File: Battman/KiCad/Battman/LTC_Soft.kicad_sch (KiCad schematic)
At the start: 14 parts, among them IC600 LTC6811IG-2#PBF, Q600 BCP56-16TF

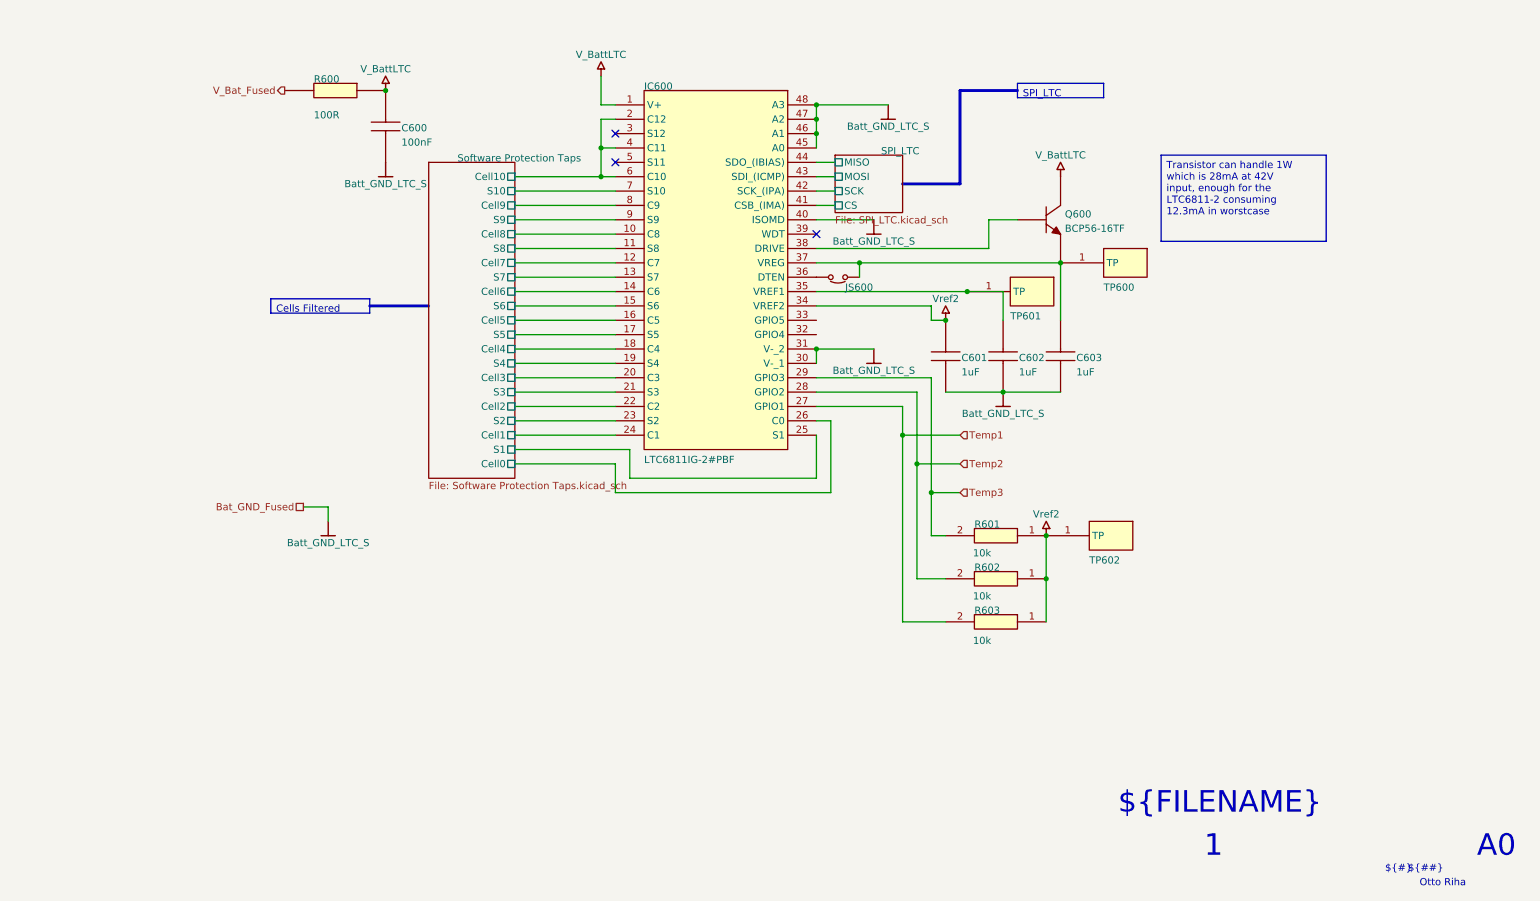
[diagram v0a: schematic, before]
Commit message: Uopdated Schematics fixed
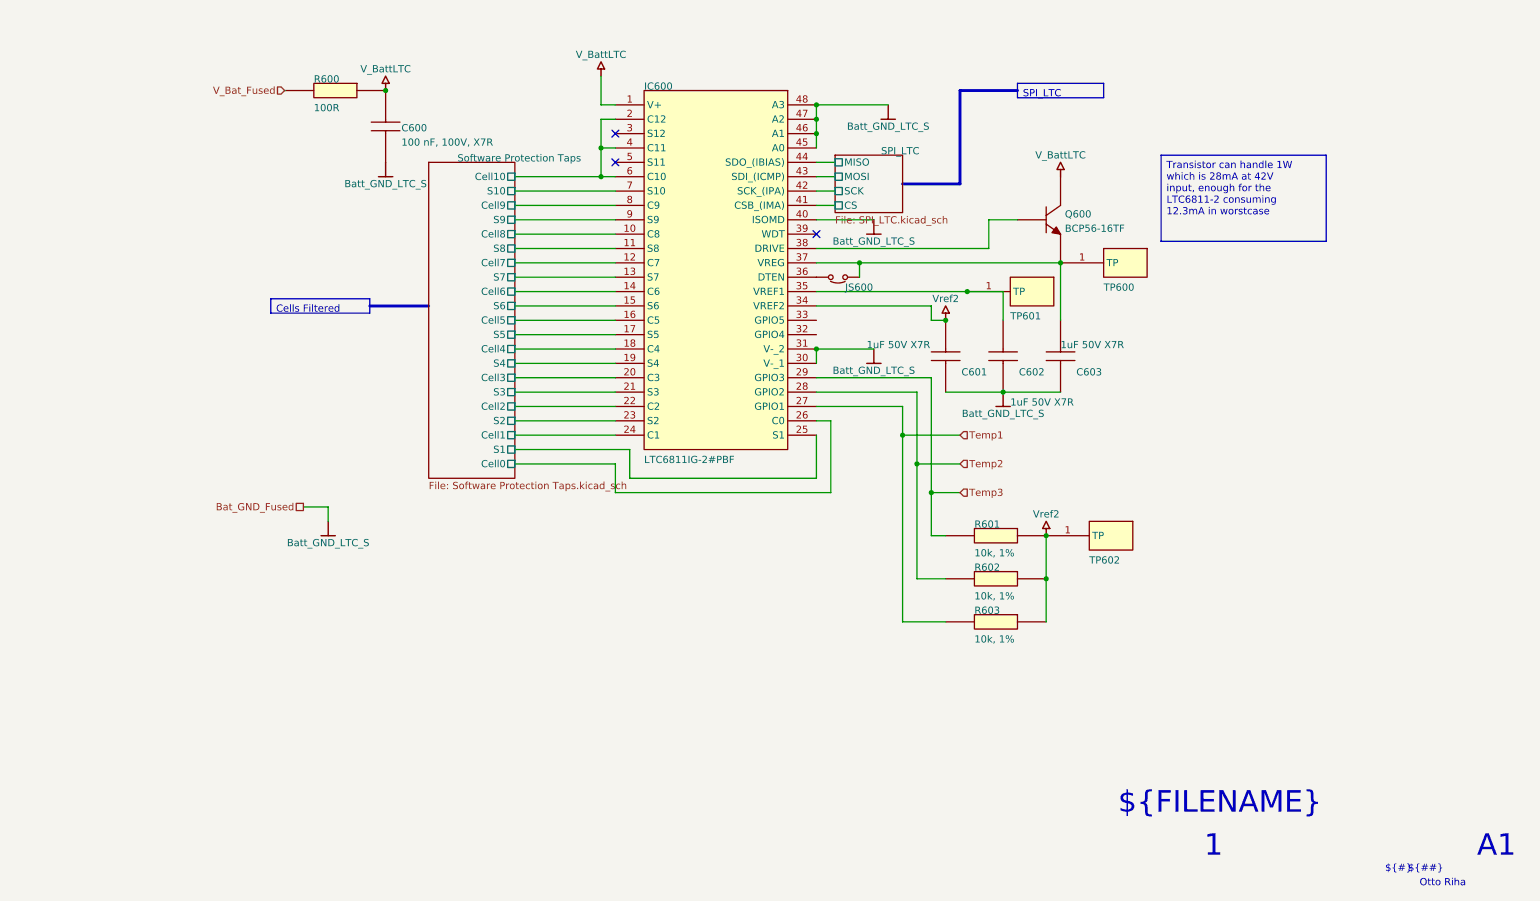
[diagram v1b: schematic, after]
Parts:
- removed C600: 0603YG104ZAT2A, C__Users_otto_Documents_AltiumLL_SamacSys.PcbLib:CAPC1608X90N, symbol Battman-altium-import:Software Protection_1_0603YG104ZAT2A_SamacSys.SchLib
- removed R601, R602, R603: CRCW060310K0FKEI, C__Users_otto_Documents_AltiumLL_SamacSys.PcbLib:RESC1608X50N, symbol Battman-altium-import:Software Protection_2_CRCW060310K0FKEI_*
- added C600: 100 nF, 100V, X7R, C__Users_otto_Documents_AltiumLL_SamacSys.PcbLib:MAJx16, symbol Battman-altium-import:Software Protection_1_MAJCH168BB7104KTEA01_SamacSys.SchLib
- added R601, R602, R603: CRCW060310K0FKEI, C__Users_otto_Documents_AltiumLL_SamacSys.PcbLib:RESC1608X50N, symbol Battman-altium-import:Software Protection_2_CRCW060310K0FKEI_SamacSys.SchLib
- C601, C602, C603: value 06035C105MAT2A -> 1uF 50V X7R
- R600: SUPPLIER 1 (none) -> Mouser; SUPPLIER PART NUMBER 1 (none) -> 71-CRCW0603-100-E3
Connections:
- net Batt_GND_LTC_S: now also C600.1
- net Temp1: now also R603.2
- net Temp2: now also R602.2
- net Temp3: now also R601.2
- net V_Bat_Fused: now also R600.1
- net V_BattLTC: now also C600.2
- net Vref2: now also R601.1, R602.1, R603.1
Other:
- note added: "A1"
- note removed: "A0"

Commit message: Begin of kicad conversion
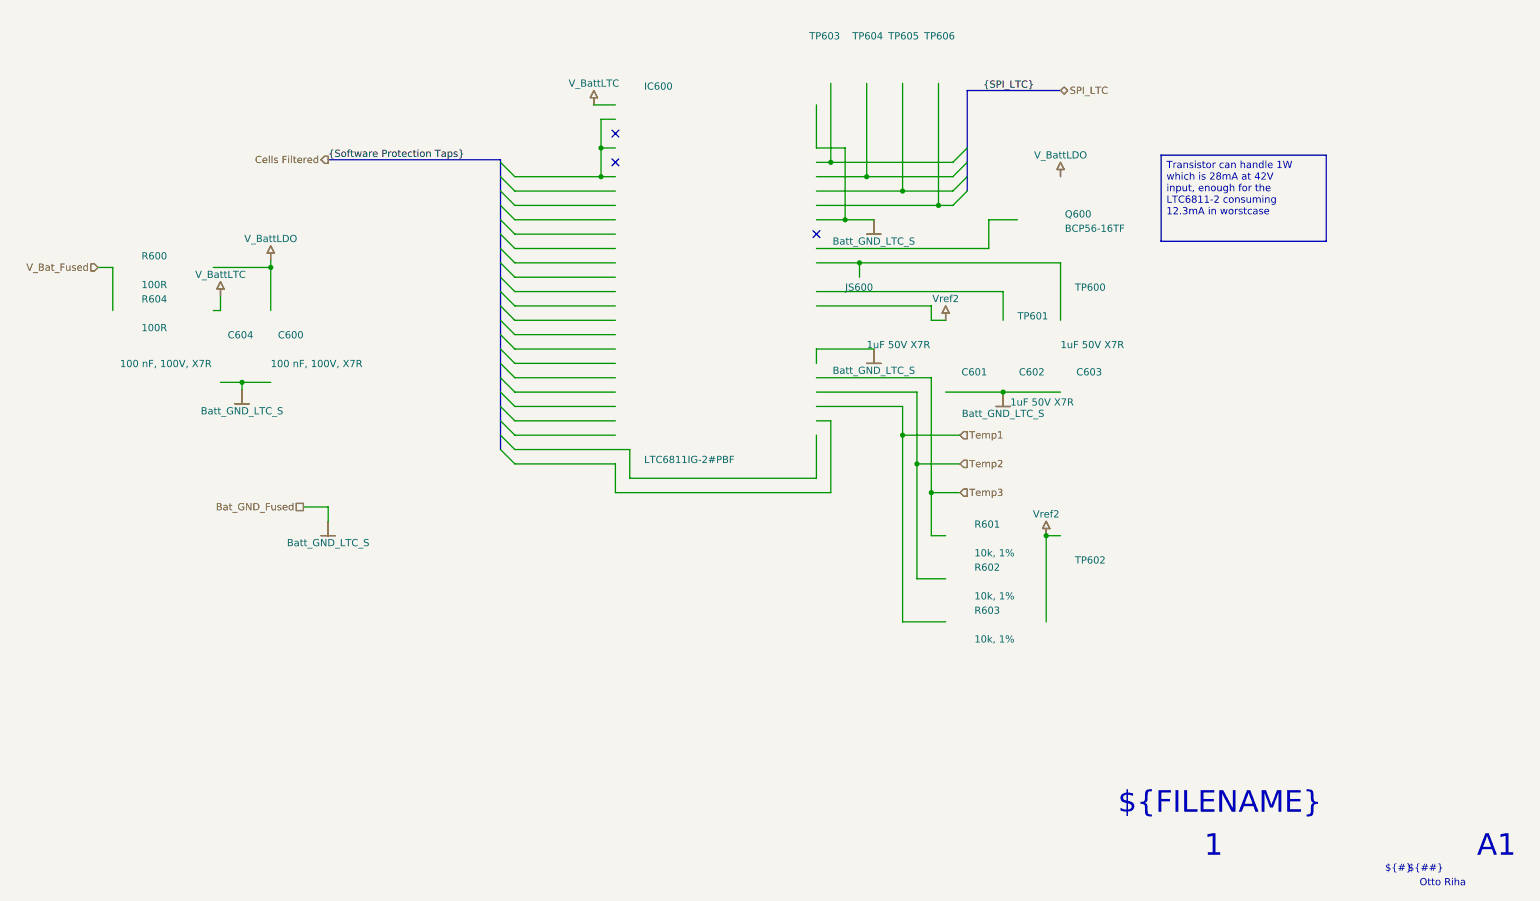
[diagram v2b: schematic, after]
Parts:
- removed C600: 100 nF, 100V, X7R, C__Users_otto_Documents_AltiumLL_SamacSys.PcbLib:MAJx16, symbol Battman-altium-import:Software Protection_1_MAJCH168BB7104KTEA01_SamacSys.SchLib
- removed C601, C602, C603: 1uF 50V X7R, C__Users_otto_Documents_AltiumLL_SamacSys.PcbLib:CAPC1608X90N, symbol Battman-altium-import:Software Protection_3_06035C105MAT2A_SamacSys.SchLib
- removed IC600: LTC6811IG-2#PBF, C__Users_otto_Documents_AltiumLL_SamacSys.PcbLib:SOP50P780X200-48N, symbol Battman-altium-import:Software Protection_0_LTC6811IG-2#PBF_*
- removed JS600: SolderJumper, SolderJumper, symbol Battman-altium-import:Software Protection_0_SolderJumper_SamacSys.SchLib
- removed Q600: BCP56-16TF, C__Users_otto_Documents_AltiumLL_SamacSys.PcbLib:SOT230P700X180-4N, symbol Battman-altium-import:Software Protection_0_BCP56-16TF_SamacSys.SchLib
- removed R600: CRCW0603100RFKEA, C__Users_otto_Documents_AltiumLL_SamacSys.PcbLib:RESC1608X50N, symbol Battman-altium-import:Software Protection_0_CRCW0603100RFKEA_SamacSys.SchLib
- removed R601, R602, R603: CRCW060310K0FKEI, C__Users_otto_Documents_AltiumLL_SamacSys.PcbLib:RESC1608X50N, symbol Battman-altium-import:Software Protection_2_CRCW060310K0FKEI_SamacSys.SchLib
- removed TP600, TP601, TP602: Test Pad 1mm, Test Pad 1mm-Footprint-1, symbol Battman-altium-import:Software Protection_0_Test Pad 1mm-Symbol-1_EPFL Racing T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
- added C600, C604: 100 nF, 100V, X7R, C__Users_otto_Documents_AltiumLL_SamacSys.PcbLib:MAJx16, symbol Battman-altium-import:Software Protection_1_MAJCH168BB7104KTEA01_SamacSys.SchLib
- added C601, C602, C603: 1uF 50V X7R, C__Users_otto_Documents_AltiumLL_SamacSys.PcbLib:CAPC1608X90N, symbol Battman-altium-import:Software Protection_3_06035C105MAT2A_SamacSys.SchLib
- added IC600: LTC6811IG-2#PBF, C__Users_otto_Documents_AltiumLL_SamacSys.PcbLib:SOP50P780X200-48N, symbol Battman-altium-import:Software Protection_0_LTC6811IG-2#PBF_*
- added JS600: SolderJumper, SolderJumper, symbol Battman-altium-import:Software Protection_0_SolderJumper_SamacSys.SchLib
- added Q600: BCP56-16TF, C__Users_otto_Documents_AltiumLL_SamacSys.PcbLib:SOT230P700X180-4N, symbol Battman-altium-import:Software Protection_0_BCP56-16TF_SamacSys.SchLib
- added R600, R604: CRCW0603100RFKEA, C__Users_otto_Documents_AltiumLL_SamacSys.PcbLib:RESC1608X50N, symbol Battman-altium-import:Software Protection_0_CRCW0603100RFKEA_SamacSys.SchLib
- added R601, R602, R603: CRCW060310K0FKEI, C__Users_otto_Documents_AltiumLL_SamacSys.PcbLib:RESC1608X50N, symbol Battman-altium-import:Software Protection_2_CRCW060310K0FKEI_SamacSys.SchLib
- added TP600, TP601, TP602: Testpoint, Testpoint, symbol Battman-altium-import:Software Protection_0_Testpoint_SamacSys.SchLib
- added TP603, TP604, TP605, TP606: Testpoint, Testpoint, symbol Battman-altium-import:Software Protection_1_Testpoint_SamacSys.SchLib
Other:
- removed sheet SPI_LTC
- removed sheet Software Protection Taps

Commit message: kicad release
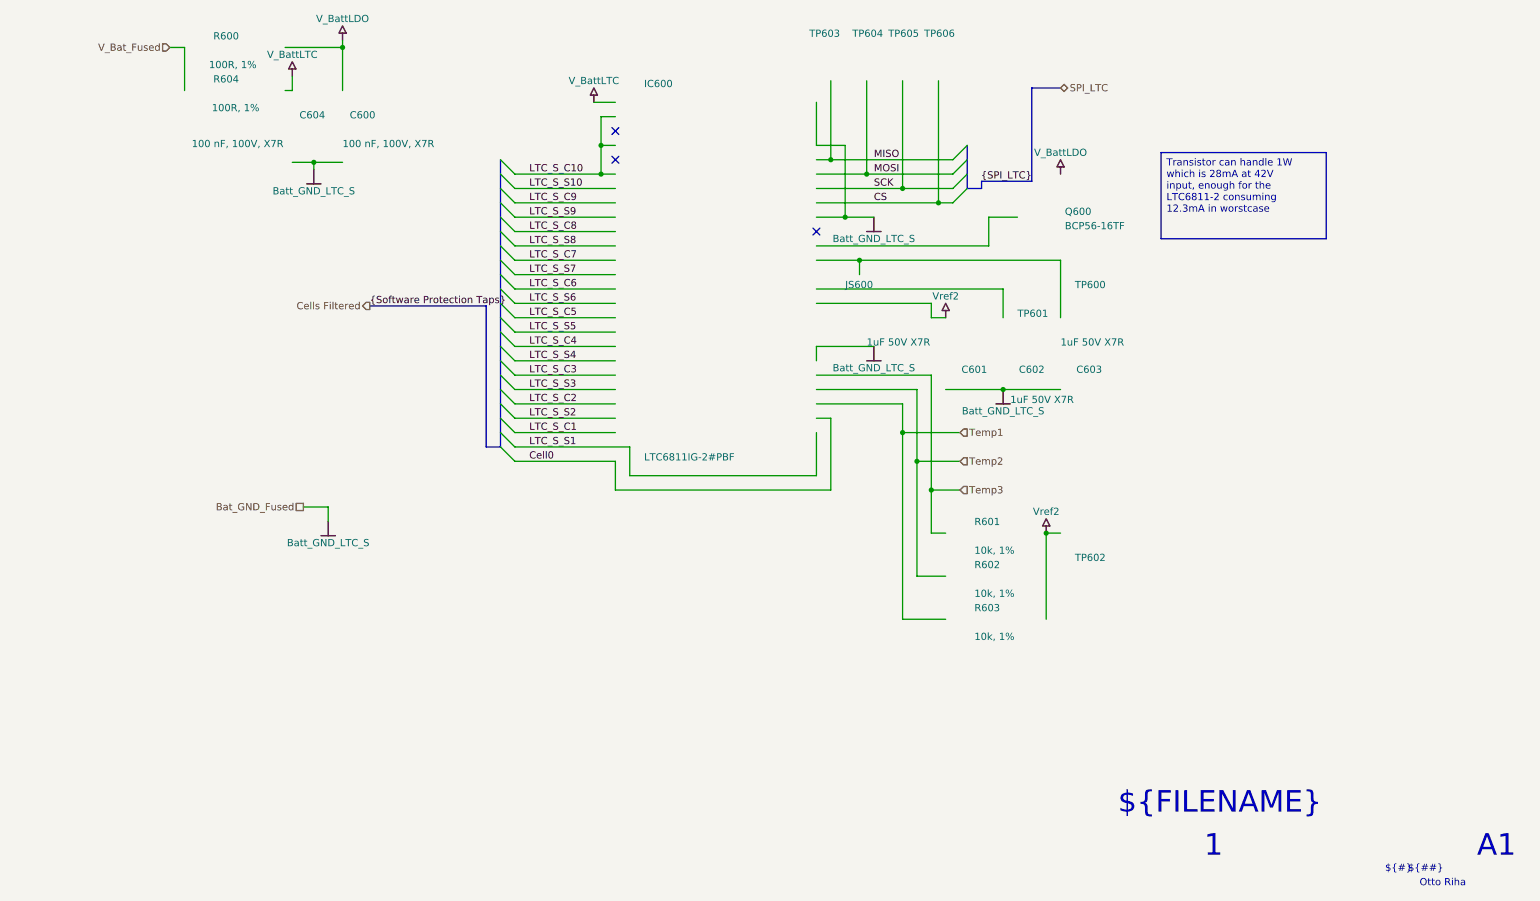
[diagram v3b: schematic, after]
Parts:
- R600, R604: value CRCW0603100RFKEA -> 100R, 1%
